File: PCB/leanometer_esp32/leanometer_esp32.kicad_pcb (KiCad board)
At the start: 4 copper layers, 95.5 x 58.5 mm, 69 parts, among them J1 Conn_01x07, J2 PROG, J3 VBAT, J4 DM3AT-SF-PEJM5, J5 Conn_01x03, J6 Conn_01x07, J7 Conn_01x03, Q1 BSS138, SW1 SW_Push, SW2 SW_Push, SW3 SW_Push, U1 LD1117S33TR_SOT223, U2 ESP32-WROOM-32D, U3 MPU-6050, U4 74HC595, U5 74HC595, U6 D168K, U7 D168K, U8 GY-521

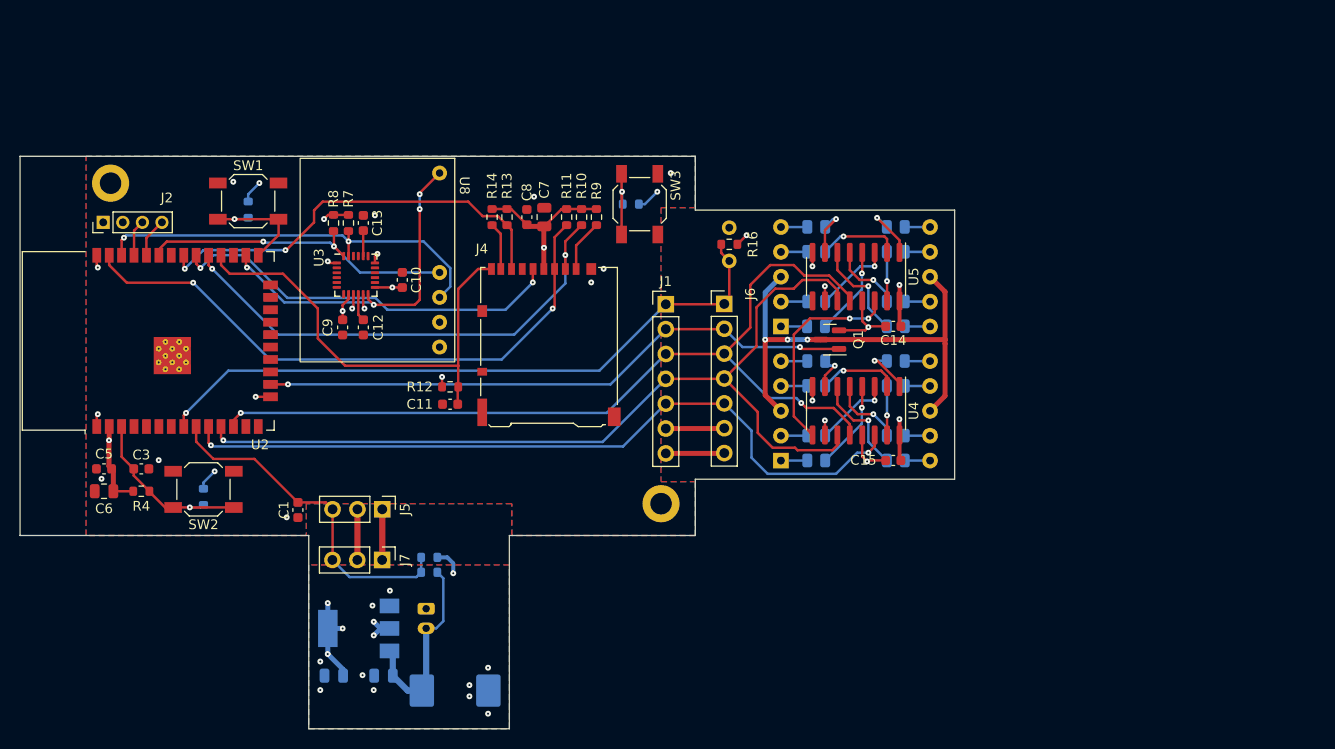
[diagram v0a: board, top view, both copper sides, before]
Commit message: Full layout rework
Signed-off-by: theloukou
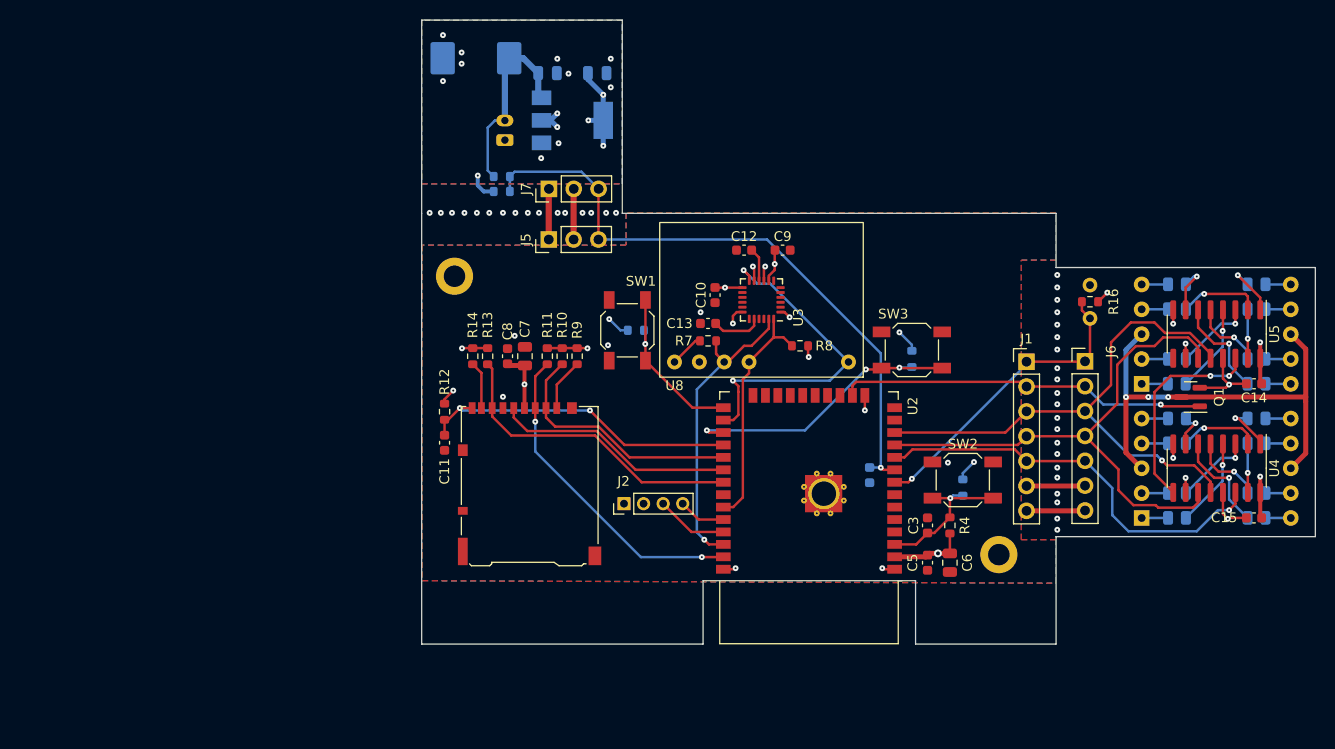
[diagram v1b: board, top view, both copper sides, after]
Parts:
- C1: moved to B.Cu
- moved C5 86.7 mm to (155.0, 117.0), turned to 90 degrees
- moved C6 84.7 mm to (152.7, 117.0), turned to -90 degrees
- moved R4 82.7 mm to (155.0, 113.2), turned to 90 degrees
- moved C3 80.5 mm to (152.7, 113.2), turned to 90 degrees
- moved R5 77.6 mm to (156.3, 109.3)
- moved SW2 77.6 mm to (156.3, 108.6)
- moved C4 67.2 mm to (119.0, 67.0), turned to 0 degrees
- moved U2 66.3 mm to (140.6, 109.4), turned to 180 degrees
- moved D1 64.7 mm to (106.6, 65.5), turned to 0 degrees
- moved C2 63.8 mm to (113.9, 67.0), turned to 0 degrees
- moved J2 60.5 mm to (121.7, 111.0)
- moved C1 58.5 mm to (146.8, 108.1)
- moved U1 56.3 mm to (116.4, 71.8), turned to 0 degrees
- moved R8 49.3 mm to (139.7, 94.9), turned to 180 degrees
- moved J3 48.6 mm to (109.5, 73.8), turned to 90 degrees
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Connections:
- U2 pad 27: unconnected-(U2-IO16-Pad27) -> /MainBoard/BUT
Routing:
- net /DisplayBoard/ADC_LDR: track 67.8 -> 31.4 mm
- net /DisplayBoard/DISP_DATA: track 78.7 -> 42.7 mm, vias 2 -> 1
- net /DisplayBoard/DISP_CLOCK: track 92.2 -> 56.6 mm, vias 1 -> 0
- net /DisplayBoard/DISP_LATCH: track 91.5 -> 58.3 mm, vias 2 -> 1
- net /MainBoard/ADC_VBAT: track 35.1 -> 64.7 mm, vias 0 -> 1
- net /MainBoard/SD_MOSI: track 61.6 -> 33.1 mm
- net /MainBoard/SD_SS: track 50.6 -> 25.9 mm, vias 2 -> 0
- net /DisplayBoard/DISP_BRIGHT: track 61.3 -> 37.8 mm, vias 2 -> 1
- net /MainBoard/BUT: track 7.54 -> 29.8 mm, vias 1 -> 3
- net /MainBoard/SD_SCK: track 40.9 -> 24.6 mm, vias 2 -> 0
- net /MainBoard/SD_DET_B: track 47.3 -> 33.4 mm, vias 0 -> 2
- net /MainBoard/SD_MISO: track 43.6 -> 31.9 mm, vias 2 -> 0
- net /MainBoard/I2C_SCL: track 42.7 -> 31.2 mm, vias 2 -> 1
- net /MainBoard/I2C_SDA: track 33.9 -> 24.8 mm, vias 2 -> 0
- net /MainBoard/IO0: track 12.2 -> 17.6 mm
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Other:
- board size 95.5 x 58.5 mm -> 91.3 x 63.8 mm
